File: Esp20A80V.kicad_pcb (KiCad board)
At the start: 2 copper layers, 75 x 29 mm, 19 parts, among them J1 dcdc, J4 I2C/Uart, Q1 SI2305, SW1 3x button, U1 spi tft with touch (+ sd card), U3 20A 80V dcdc, U4 Wemos S2 Mini

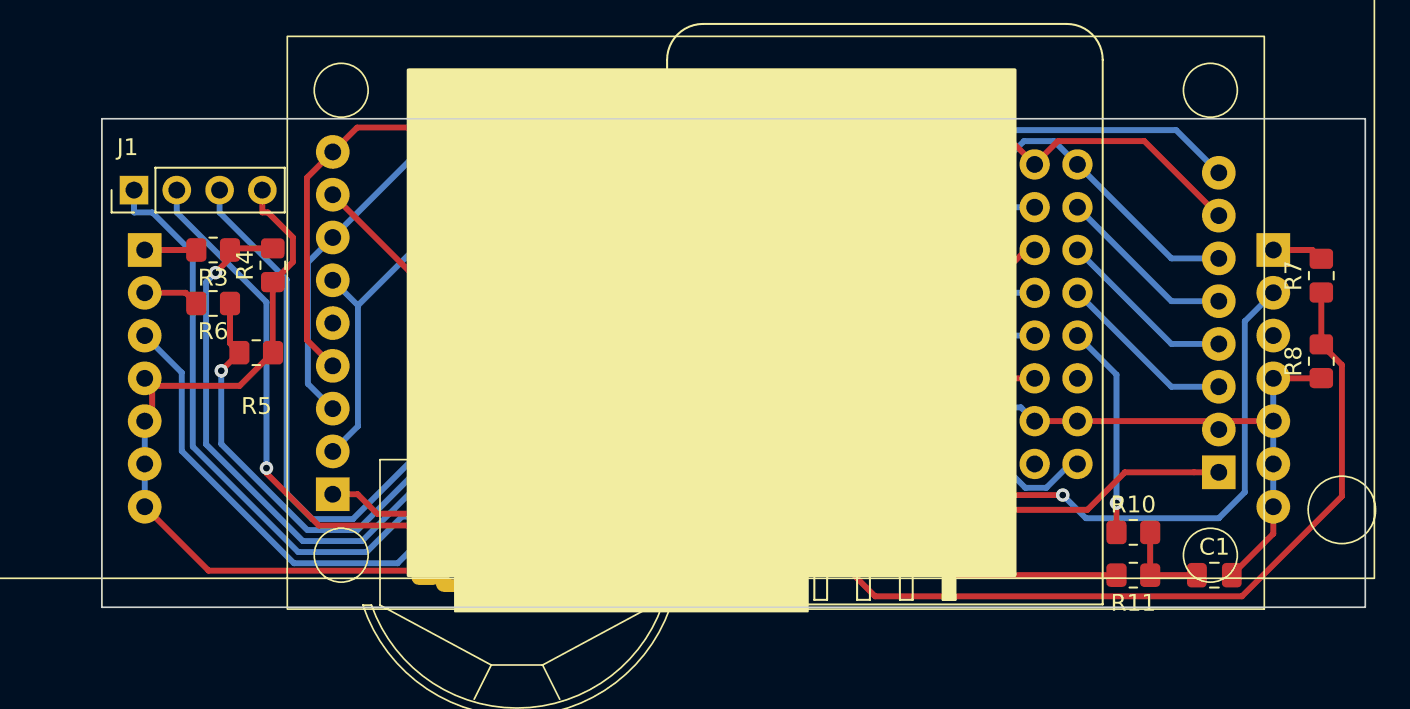
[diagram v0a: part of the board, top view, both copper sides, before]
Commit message: better circuit
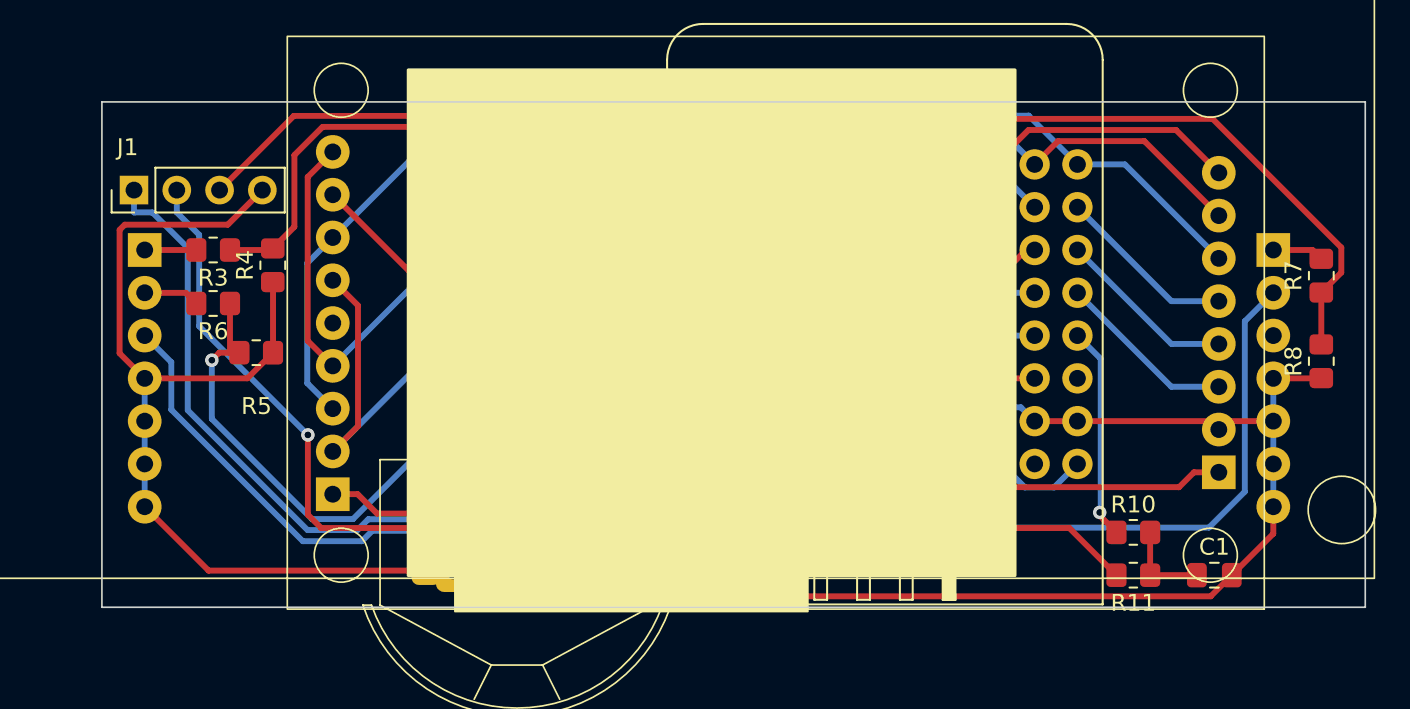
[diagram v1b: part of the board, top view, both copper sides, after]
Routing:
- net GND: track 118.4 -> 146.1 mm
- net iVout: track 74.7 -> 47.6 mm, vias 1 -> 0
- net enable: track 53.1 -> 36.0 mm, vias 1 -> 0
- net +5V: track 96.6 -> 102.8 mm
- net SCK: track 70.5 -> 75.7 mm
- net MISO: track 57.3 -> 62.5 mm
- net DAC in: track 64.3 -> 61.8 mm
- net mode: track 54.3 -> 52.1 mm
- net Iout: track 54.4 -> 55.7 mm, vias 1 -> 0
- net Net-(U1-VCC): track 33.3 -> 32.2 mm
- net Net-(Q1-S): track 20.9 -> 20.1 mm, vias 1 -> 0
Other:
- board size 75 x 29 mm -> 75 x 30 mm
